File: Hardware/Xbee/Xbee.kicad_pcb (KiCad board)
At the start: 2 copper layers, 100 x 50 mm, 53 parts, among them J1 Alimentación, J2 Raspberry, J3 Pines 1, J4 Pines 2, J5 Programación, J6 Entrada, J7 Salida, J8 Batería, K1 SANYOU_SRD_Form_C, Q1 2N7002, Q2 AP2300, Q3 DMP3099L-7, SW1 Reset, SW2 Comm., U1 AZ1117-3.3, U2 Xbee, U3 LM358

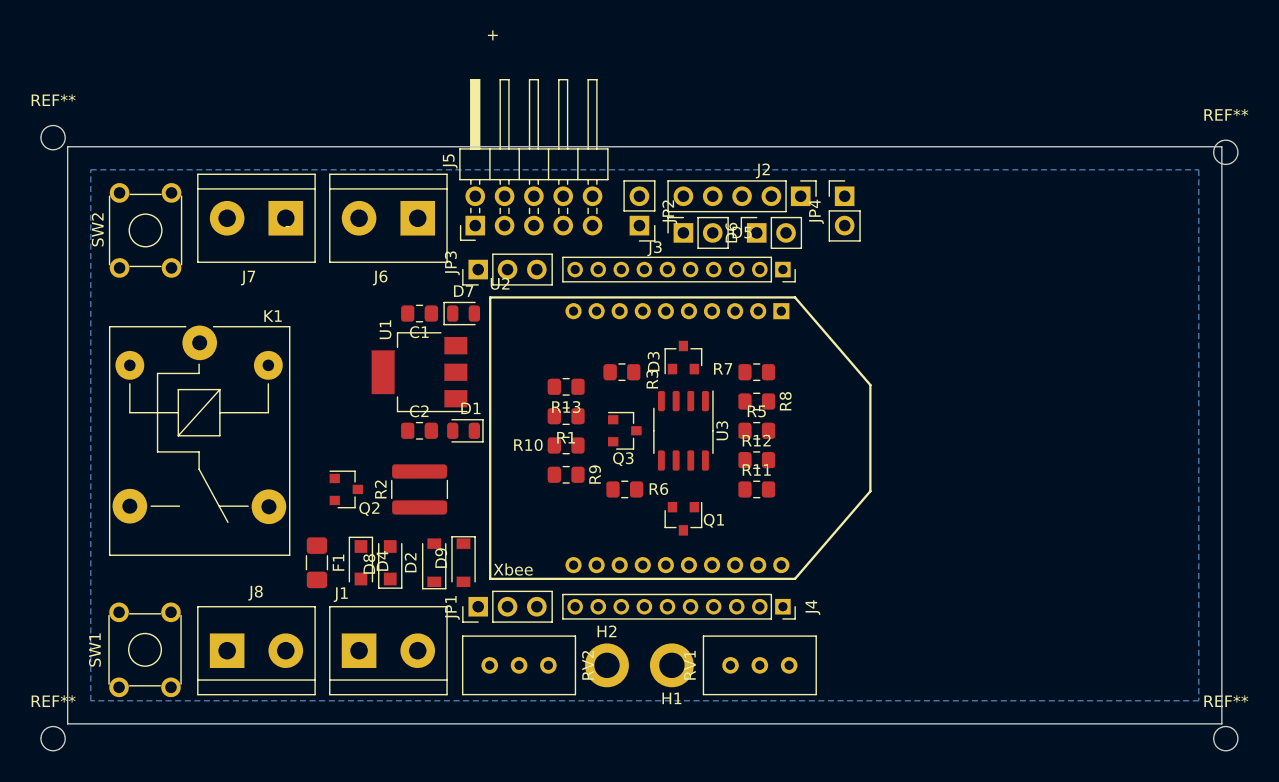
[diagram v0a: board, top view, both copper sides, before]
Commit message: Comienzo de ruteo
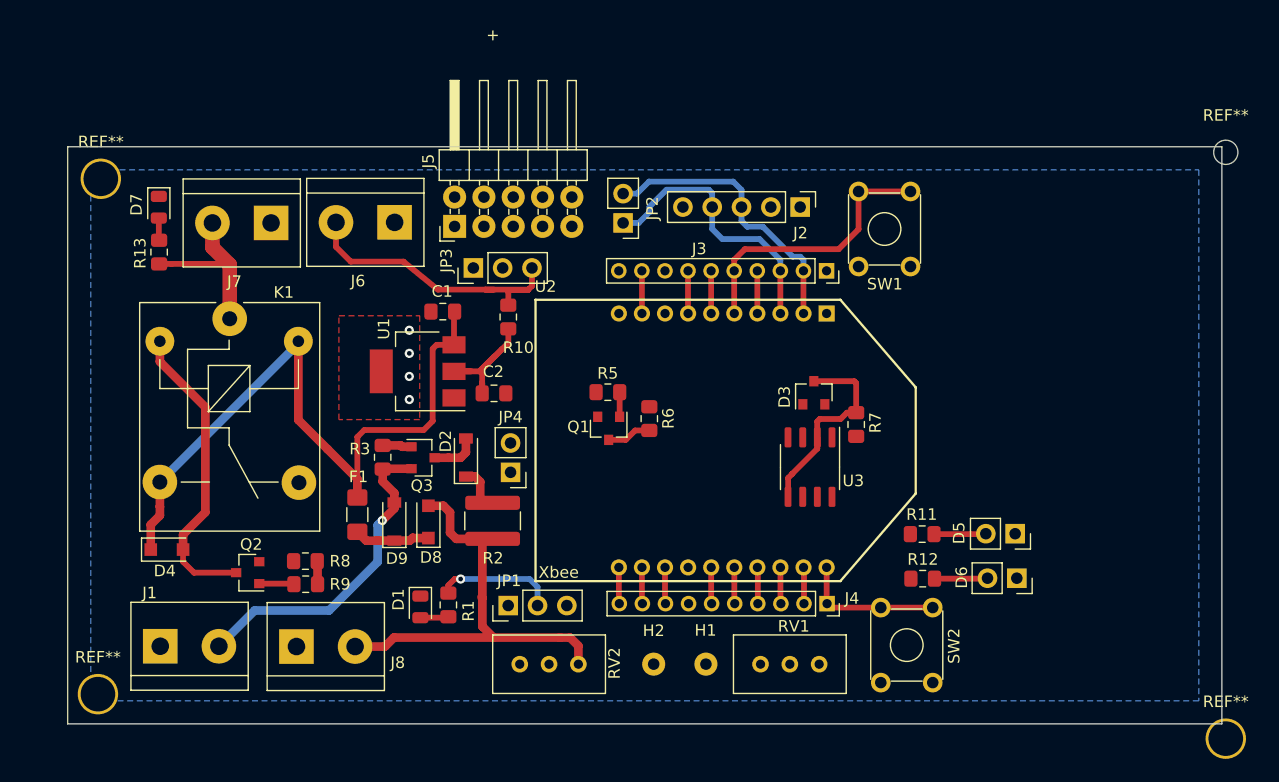
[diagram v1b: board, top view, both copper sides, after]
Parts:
- moved SW2 74.7 mm to (150.4, 76.4), turned to 90 degrees
- moved SW1 73.7 mm to (148.5, 40.4)
- moved R8 41.5 mm to (100.6, 65.9), turned to 180 degrees
- moved D5 38.8 mm to (162.1, 63.5), turned to 270 degrees
- moved JP4 37.5 mm to (118.4, 58.2), turned to 180 degrees
- moved D6 37.5 mm to (162.2, 67.4), turned to 270 degrees
- moved R13 37.1 mm to (87.9, 39.1), turned to 90 degrees
- moved D7 28.0 mm to (87.9, 35.2), turned to 270 degrees
- moved R9 24.5 mm to (100.6, 67.9), turned to 0 degrees
- moved R3 22.0 mm to (107.3, 56.9), turned to 90 degrees
- moved R1 19.3 mm to (113.0, 69.7), turned to 90 degrees
- moved R12 17.7 mm to (154.1, 67.4), turned to 180 degrees
- moved Q3 17.6 mm to (110.8, 56.9)
- moved J1 17.2 mm to (88.0, 73.3)
- moved D4 16.8 mm to (88.6, 64.9), turned to 0 degrees
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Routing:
- net +12V: track 0.00 -> 60.8 mm
- net /Bat+: track 0.00 -> 38.3 mm
- net /Vin+: track 0.00 -> 28.9 mm, vias 0 -> 1
- net /Bobina: track 0.00 -> 26.5 mm
- net /DIO2-Entrada: track 0.00 -> 25.9 mm
- net /RXD: track 0.00 -> 25.1 mm
- net /RST: track 0.00 -> 24.3 mm
- net /TXD: track 0.00 -> 24.1 mm
- net Net-(D3-Pad1): track 0.00 -> 17.4 mm
- net /Salida-Rele: track 0.00 -> 15.1 mm
- net +3V3: track 0.00 -> 14.3 mm, vias 0 -> 4
- net /Comm.: track 0.00 -> 12.5 mm
- net /LED-Assoc-RSSI: track 0.00 -> 10.5 mm, vias 0 -> 1
- net Net-(D8-Pad1): track 0.00 -> 6.59 mm
- net Net-(D5-Pad2): track 0.00 -> 4.82 mm
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- added copper zone on F.Cu, net +3V3
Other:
- board text removed: "-"
